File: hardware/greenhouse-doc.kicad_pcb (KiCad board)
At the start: 2 copper layers, 64.6 x 23 mm, 34 parts, among them IC1 SC810ULTRT, IC2 TPS564247DRLR, J1 USB_B_Micro, J2 Conn_02x03_Odd_Even, J3 Conn_01x02, J4 Conn_01x02, J5 Conn_01x02, K1 ADW1203HLW, Q1 2N7002, Q2 2N7002, U1 ESP32-WROOM-32, U2 DS18B20

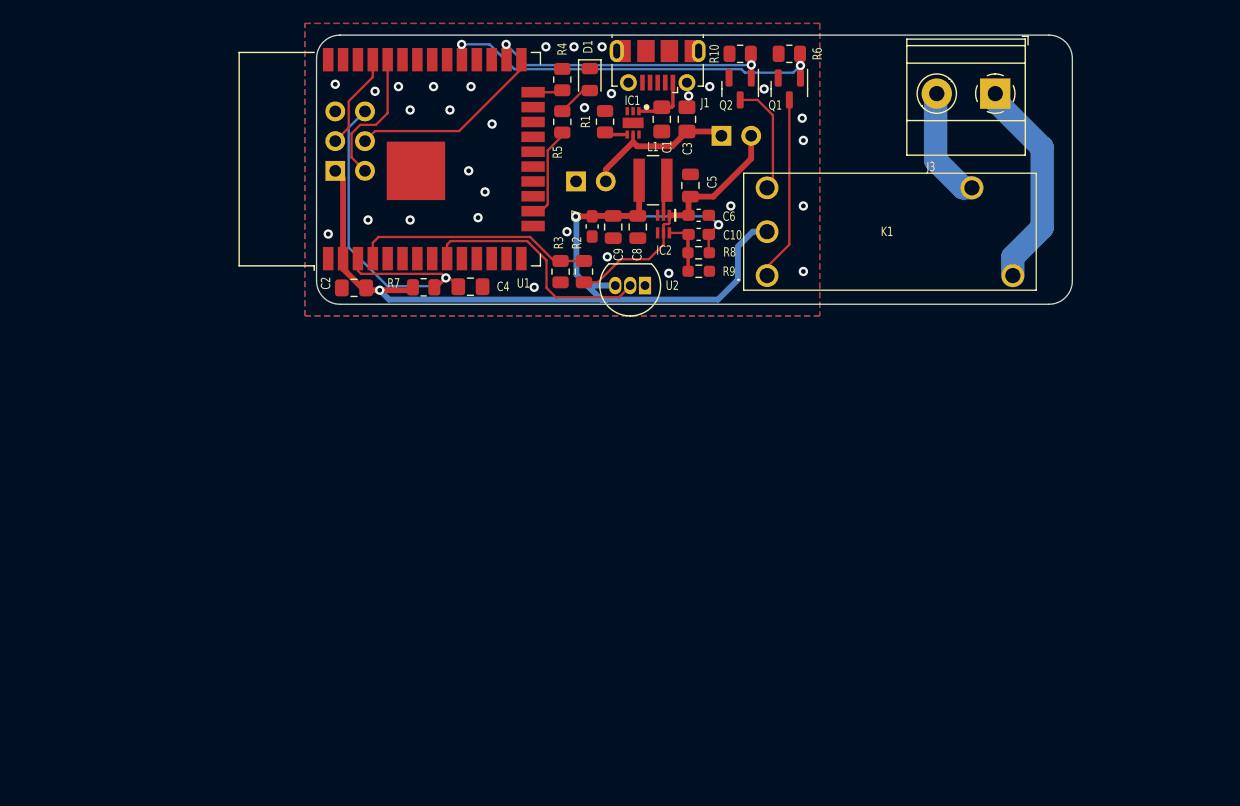
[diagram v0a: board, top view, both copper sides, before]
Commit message: v2 hardware
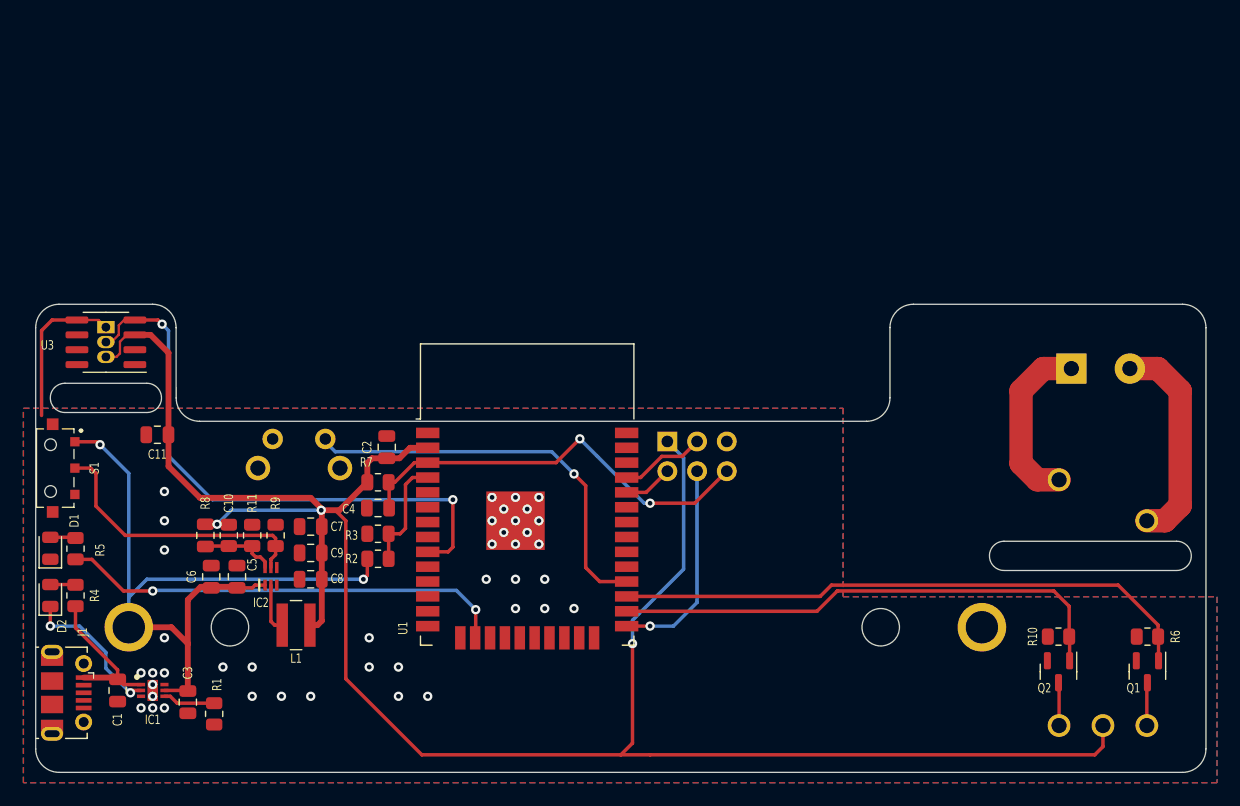
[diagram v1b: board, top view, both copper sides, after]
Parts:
- removed J4, J5: Conn_01x02, Connector_PinHeader_2.54mm:PinHeader_1x02_P2.54mm_Vertical
- added BT1: BH-18650-PC, SamacSys_Parts:BH18650PC, B.Cu at (149.9, 106.6)
- added C11: 10u, Capacitor_SMD:C_0805_2012Metric, F.Cu at (79.4, 90.2)
- added D2: LED, LED_SMD:LED_0805_2012Metric, F.Cu at (70.2, 103.9)
- added R11: 10k, Resistor_SMD:R_0805_2012Metric, F.Cu at (89.5, 98.8)
- added S1: JS102000SAQN, SamacSys_Parts:JS102000SAQN, F.Cu at (72.8, 93.0)
- added SW1: SW_SPST, Button_Switch_THT:SW_Tactile_SPST_Angled_PTS645Vx58-2LFS, B.Cu at (93.8, 90.5)
- added U3: DS18B20Z, Package_SO:SOIC-8_3.9x4.9mm_P1.27mm, F.Cu at (75.0, 82.2)
- C1, C2, C3, C4: footprint Capacitor_SMD:C_0805_2012Metric_Pad1.18x1.45mm_HandSolder -> Capacitor_SMD:C_0805_2012Metric
- C10, C6, C7: footprint Capacitor_SMD:C_0603_1608Metric_Pad1.08x0.95mm_HandSolder -> Capacitor_SMD:C_0805_2012Metric
- J3, K1, U2: moved to B.Cu
- R4: value 10k -> 1k
- R8: value 100k -> 120k; footprint Resistor_SMD:R_0603_1608Metric_Pad0.98x0.95mm_HandSolder -> Resistor_SMD:R_0805_2012Metric
- R9: value 22k -> 30k; footprint Resistor_SMD:R_0603_1608Metric_Pad0.98x0.95mm_HandSolder -> Resistor_SMD:R_0805_2012Metric
- moved J1 73.7 mm to (71.6, 112.2), turned to -90 degrees
- moved C1 67.4 mm to (76.0, 112.0)
- moved C3 65.6 mm to (82.0, 113.0), turned to -90 degrees
- moved IC1 63.5 mm to (79.0, 112.0), turned to 0 degrees
- moved D1 61.1 mm to (70.2, 99.8), turned to 90 degrees
- moved R1 60.6 mm to (84.2, 114.0), turned to 90 degrees
- moved R4 60.6 mm to (72.4, 103.9)
- moved Q1 58.4 mm to (164.0, 110.4)
- moved R6 58.4 mm to (164.0, 107.4)
- moved Q2 56.7 mm to (156.4, 110.4)
- moved R10 56.7 mm to (156.4, 107.4)
- moved R5 55.3 mm to (72.4, 99.9)
- moved C6 51.9 mm to (84.0, 102.3), turned to 90 degrees
- moved C5 51.2 mm to (86.2, 102.3)
- moved C10 49.4 mm to (83.5, 98.8), turned to -90 degrees
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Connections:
- C1 pad 1: Net-(C1-Pad1) -> +5V
- C5 pad 1: /vbt -> +BATT
- C6 pad 1: /vbt -> +BATT
- IC1 pad 1: Net-(C1-Pad1) -> +5V
- IC1 pad 2: unconnected-(IC1-Pad2) -> Net-(D2-K)
- IC2 pad 1: /vbt -> +BATT
- IC2 pad 5: /vbt -> /pw_en
- J1 pad 1: Net-(C1-Pad1) -> +5V
- K1 pad 1: Net-(K1-Pad1) -> Net-(K1-COIL-_1)
- K1 pad 6: Net-(K1-Pad6) -> Net-(K1-COIL-_2)
- Q1 pad 3: Net-(K1-Pad1) -> Net-(K1-COIL-_2)
- Q2 pad 3: Net-(K1-Pad6) -> Net-(K1-COIL-_1)
- R2 pad 2: /vbt -> +BATT
- R4 pad 1: GND -> Net-(D2-A)
- R4 pad 2: Net-(R4-Pad2) -> +5V
- U1 pad 24: Net-(R4-Pad2) -> unconnected-(U1-IO2-Pad24)
- U1 pad 27: unconnected-(U1-Pad27) -> /relay_2
- U1 pad 28: unconnected-(U1-Pad28) -> Net-(SW1-A)
- U1 pad 29: /relay_2 -> unconnected-(U1-IO5-Pad29)
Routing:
- net +3V3: track 87.5 -> 181.1 mm
- net +BATT: track 13.3 -> 64.0 mm, vias 0 -> 2
- net Net-(SW1-A): track 0.00 -> 34.8 mm, vias 0 -> 1
- net Net-(U1-IO13): track 8.15 -> 38.4 mm, vias 0 -> 2
- net /tempsens: track 20.8 -> 49.9 mm, vias 0 -> 2
- net /vbt: track 24.4 -> 0.00 mm
- net /pw_en: track 0.00 -> 23.9 mm
- net /relay_1: track 25.1 -> 43.7 mm, vias 2 -> 0
- net /relay_2: track 33.6 -> 50.3 mm, vias 2 -> 0
- net Net-(K1-Pad1): track 15.8 -> 0.00 mm
- net GND: track 0.00 -> 13.4 mm, vias 31 -> 41
- net +5V: track 0.00 -> 12.8 mm
- net Net-(D2-K): track 0.00 -> 12.7 mm, vias 0 -> 2
- net /batt_status: track 20.5 -> 9.66 mm
- net Net-(K1-Pad6): track 9.75 -> 0.00 mm
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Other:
- board size 64.6 x 23 mm -> 100 x 40 mm
- board text removed: "BATT+"
- board text removed: "GND"
